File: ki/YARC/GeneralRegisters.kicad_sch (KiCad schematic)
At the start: 13 parts, among them U71 74LS670, U72 74LS670, U73 74LS157, U74 74LS670, U75 74LS670, U76 74LS157, U77 74LS670, U78 74LS670, U79 74LS157, U80 74LS670, U81 74LS670, U82 74LS157, U96 74LS32

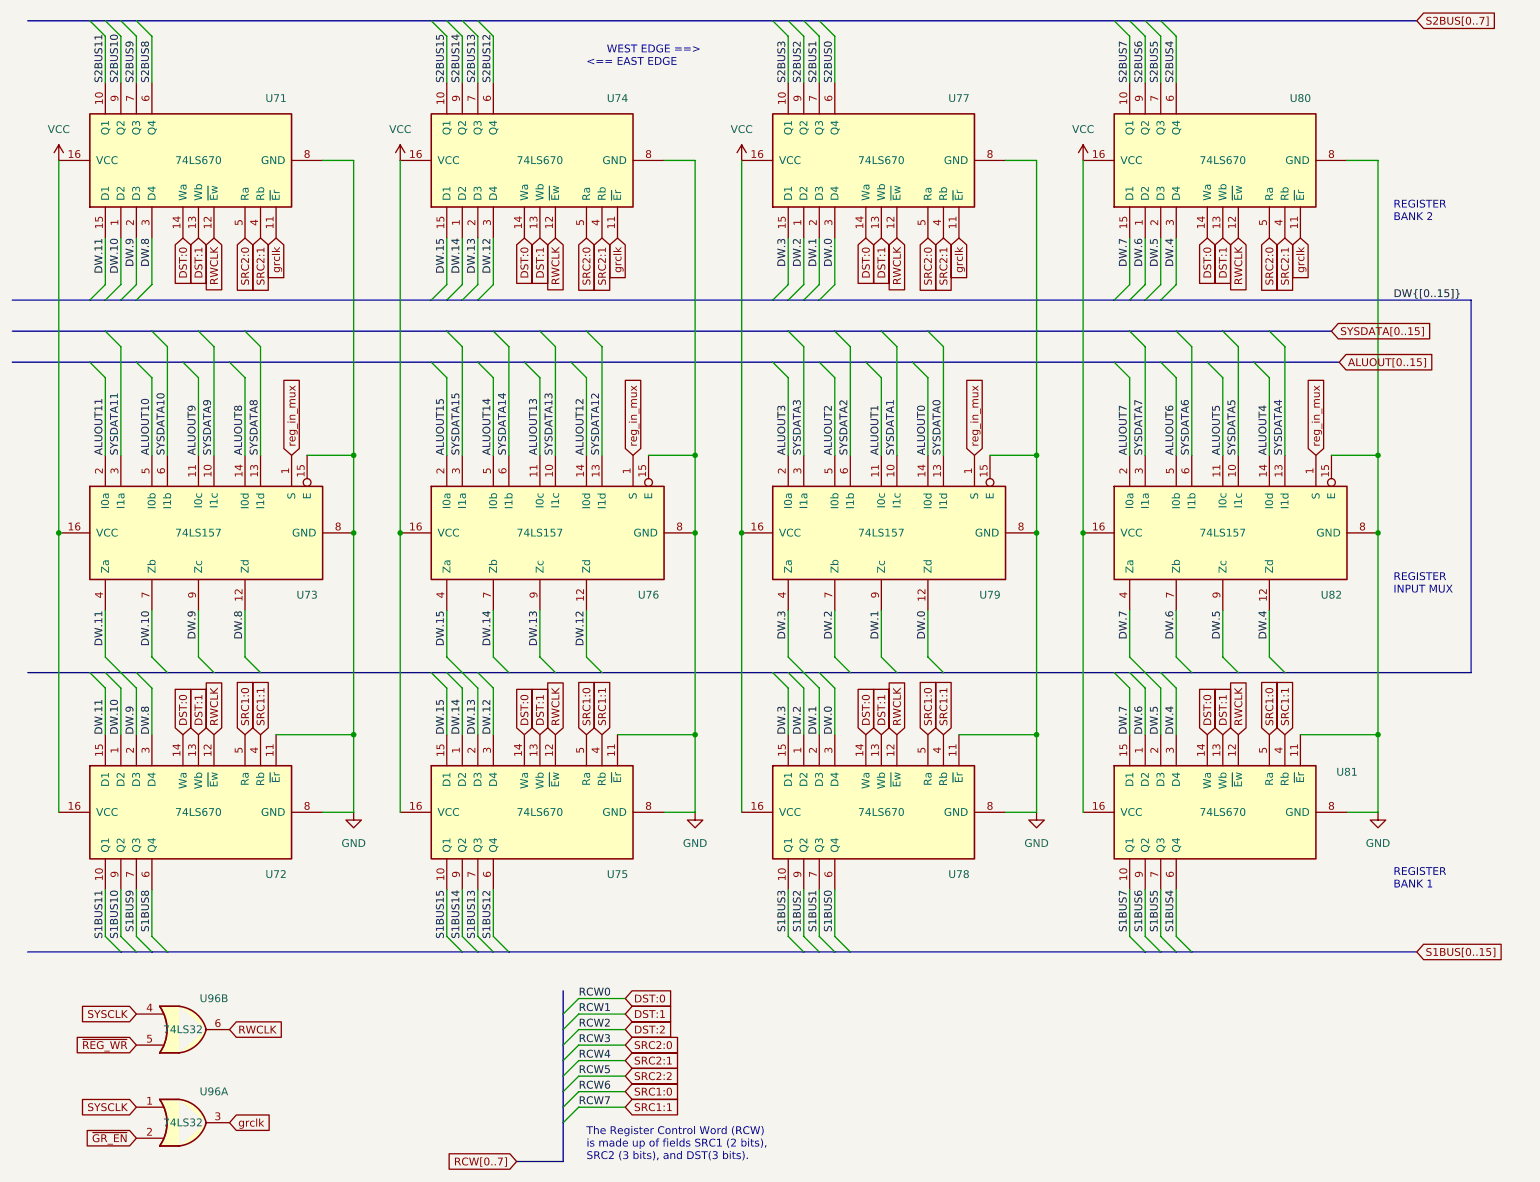
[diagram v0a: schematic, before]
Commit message: Ongoing schematic changes
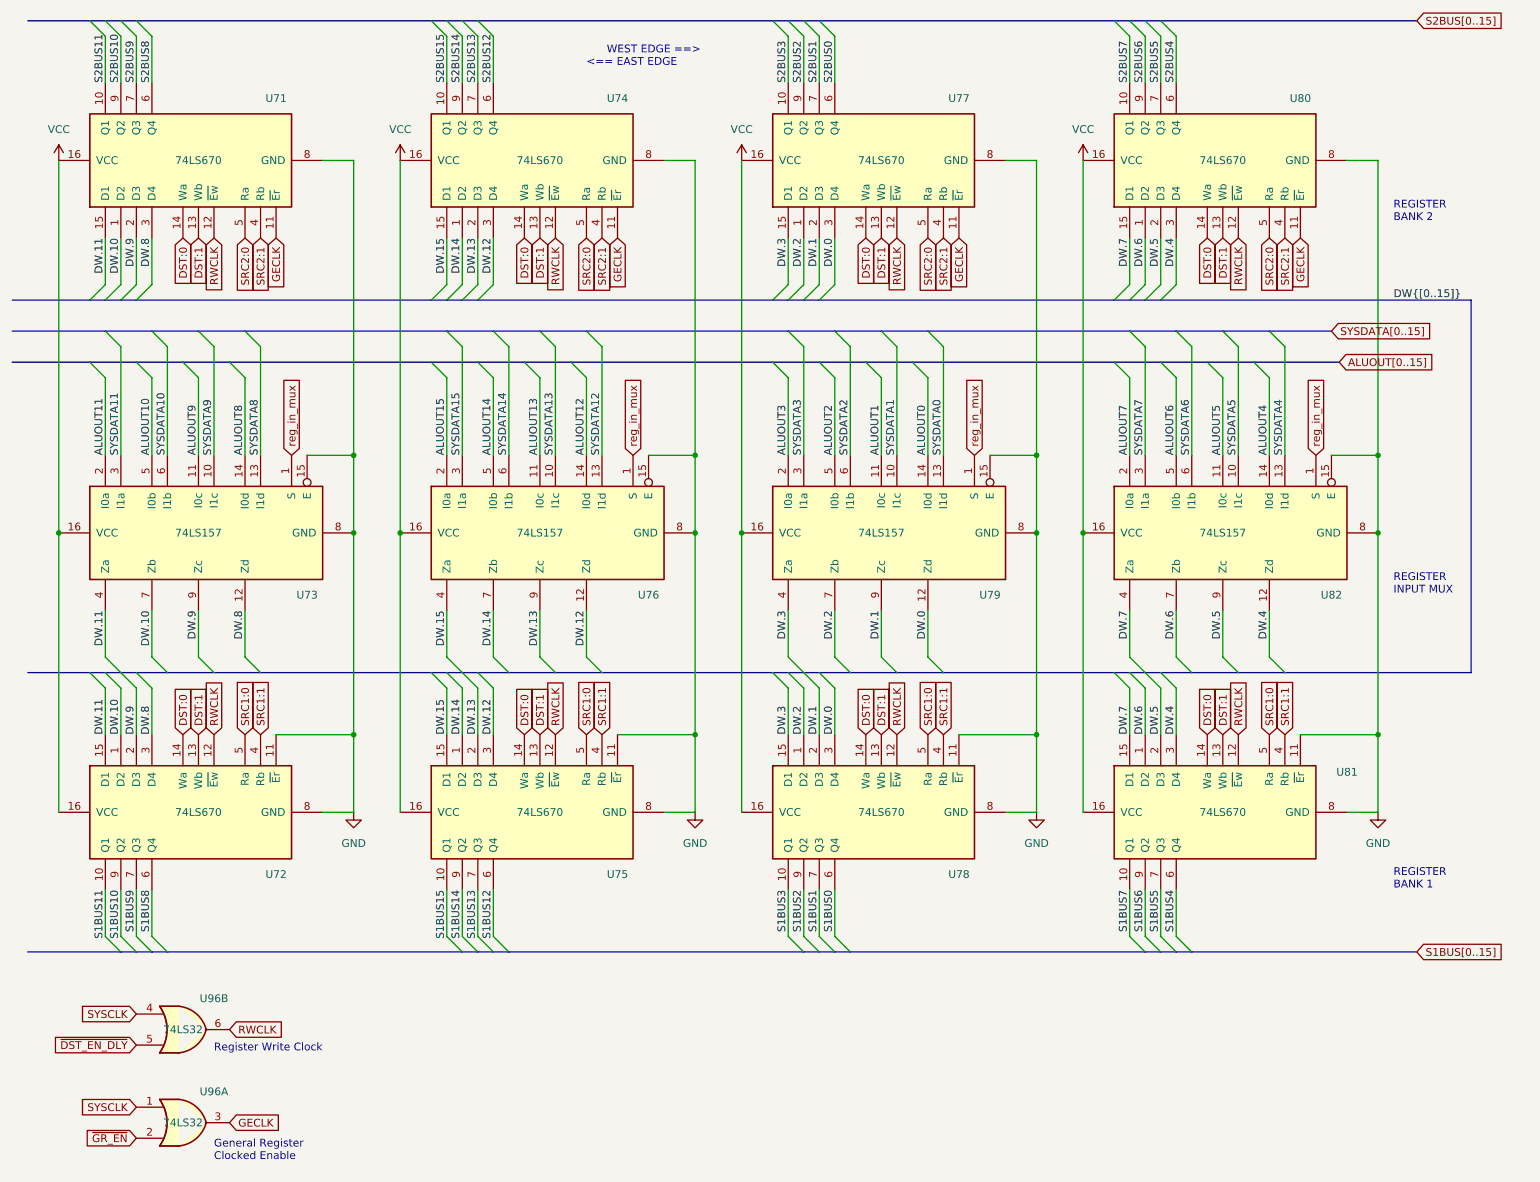
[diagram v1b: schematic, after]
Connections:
- net grclk renamed GECLK
- net ~{REG_WR} renamed ~{DST_EN_DLY}
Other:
- note added: "General Register Clocked Enable"
- note added: "Register Write Clock"
- note removed: "The Register Control Word (RCW) is made up of fields SRC1 (2 bits), SRC2 (3 bits), and DST(3 bits)."
